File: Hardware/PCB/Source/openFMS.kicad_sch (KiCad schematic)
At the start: 47 parts, among them U1 STM32F030F4Px, X1 8 MHz

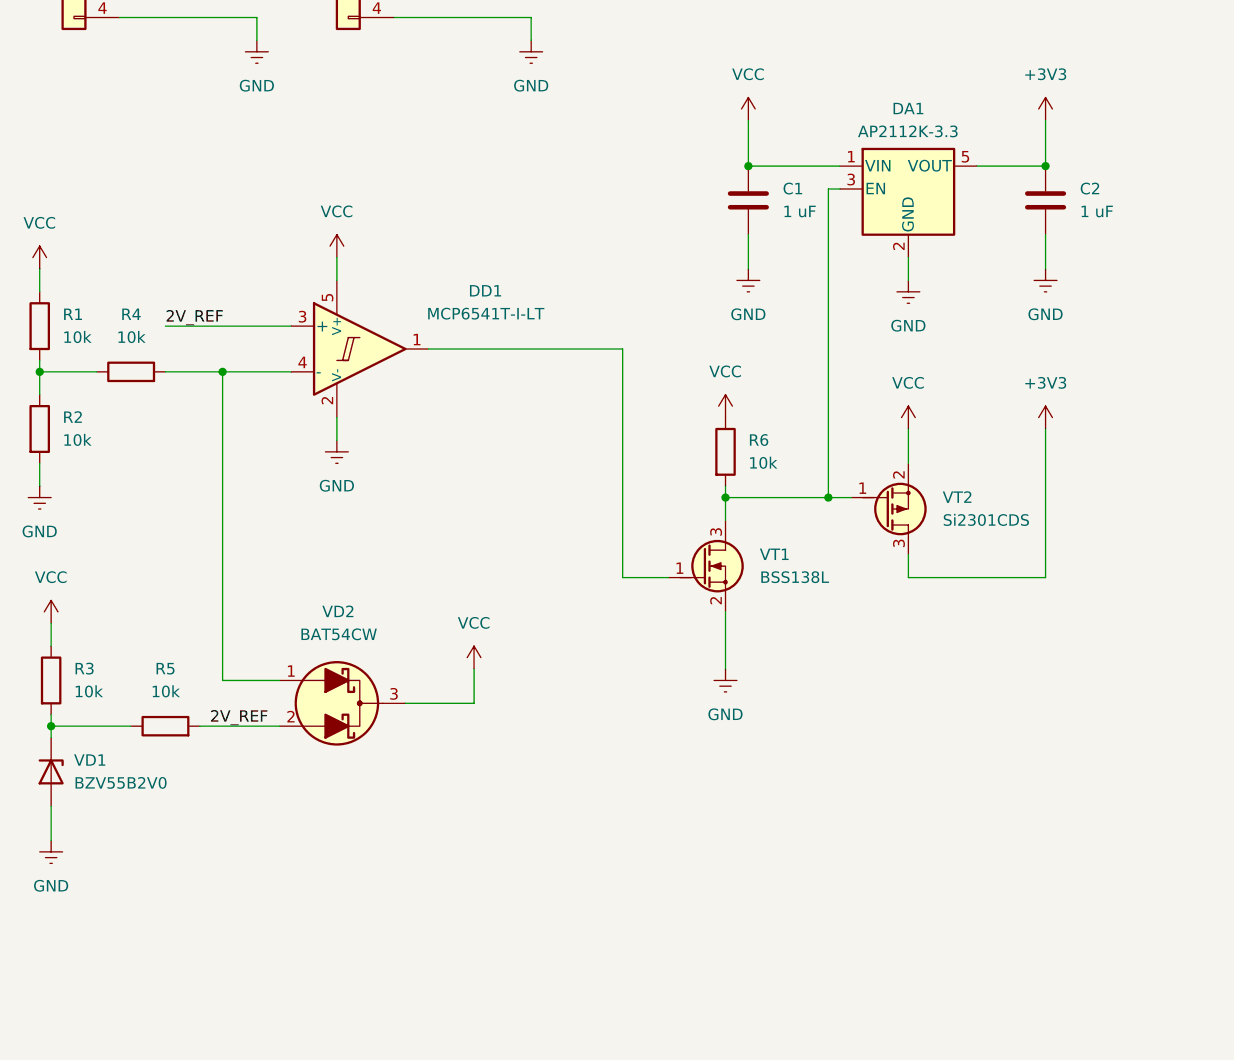
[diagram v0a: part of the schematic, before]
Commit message: WIP: routing
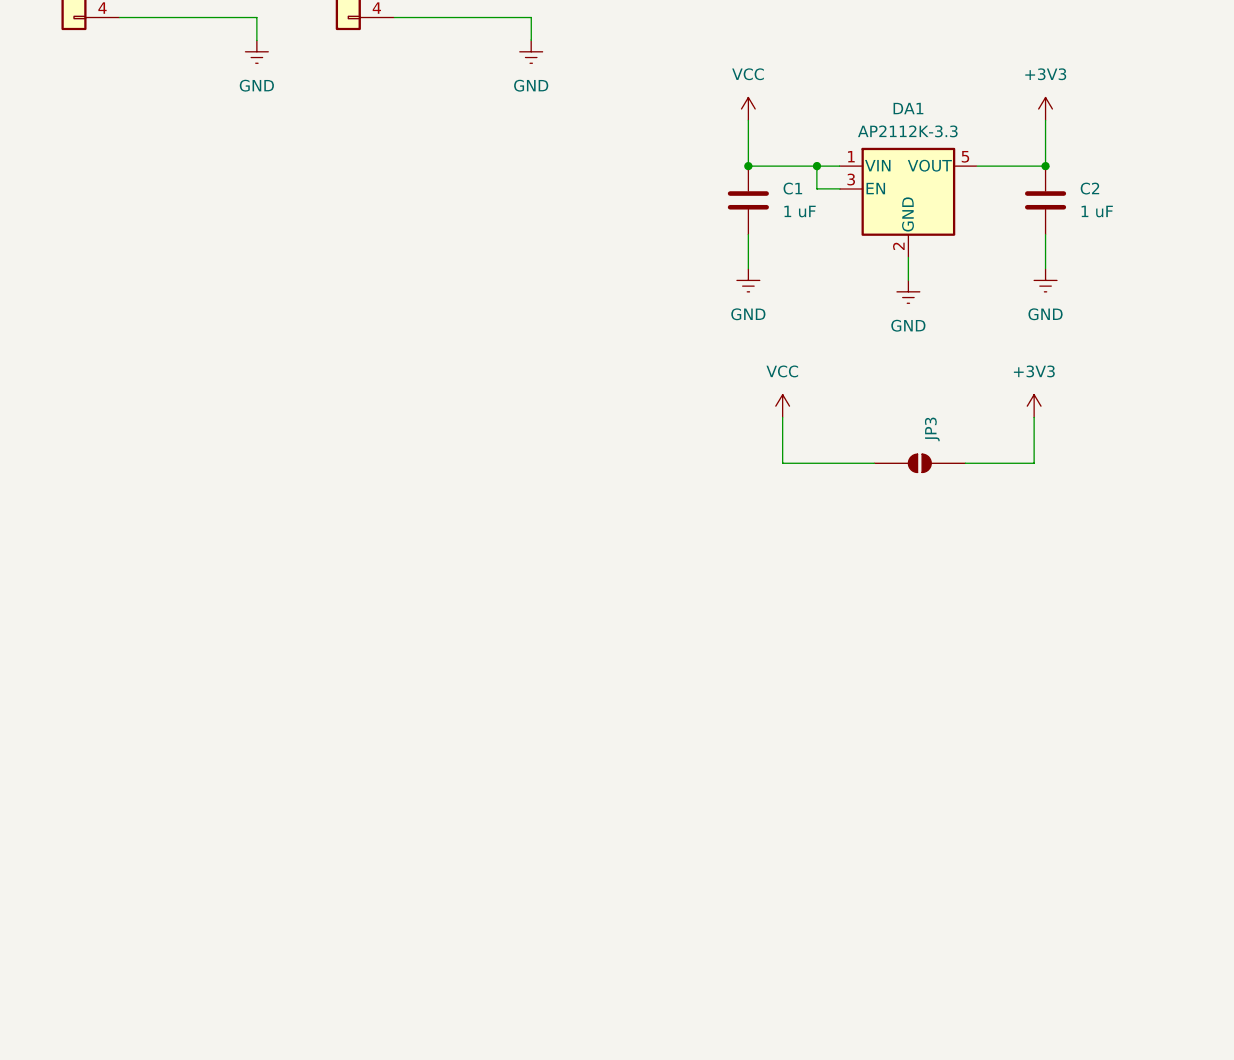
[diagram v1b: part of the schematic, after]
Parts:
- removed DD1: MCP6541T-I-LT, Package_TO_SOT_SMD_AKL:SOT-353_SC-70-5, symbol Analog_Comparator_AKL:MCP6541T-I-LT
- removed R1, R2, R3, R4, R5, R6: 10k, Resistor_SMD:R_0603_1608Metric, symbol Device:R
- removed VD1: BZV55B2V0, Diode_SMD:D_MiniMELF, symbol Diode:BZV55B2V4
- removed VD2: BAT54CW, Package_TO_SOT_SMD_AKL:SOT-323_SC-70, symbol Diode_Schottky_AKL:BAT54CW
- removed VT1: BSS138L, Package_TO_SOT_SMD_AKL:SOT-23, symbol Transistor_MOSFET_AKL:BSS138L
- removed VT2: Si2301CDS, Package_TO_SOT_SMD_AKL:SOT-23, symbol Transistor_MOSFET_AKL:Si2301CDS
- added JP3: SolderJumper_2_Open, Jumper:SolderJumper-2_P1.3mm_Open_TrianglePad1.0x1.5mm, symbol Jumper:SolderJumper_2_Open
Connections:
- net +3V3: now also JP3.2 (B)
- net VCC: now also DA1.3 (EN), JP3.1 (A)
